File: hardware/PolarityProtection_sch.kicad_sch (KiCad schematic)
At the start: 14 parts, among them IC1 LM74502HDDFR, Q4 PSMN8R5-40MSDX

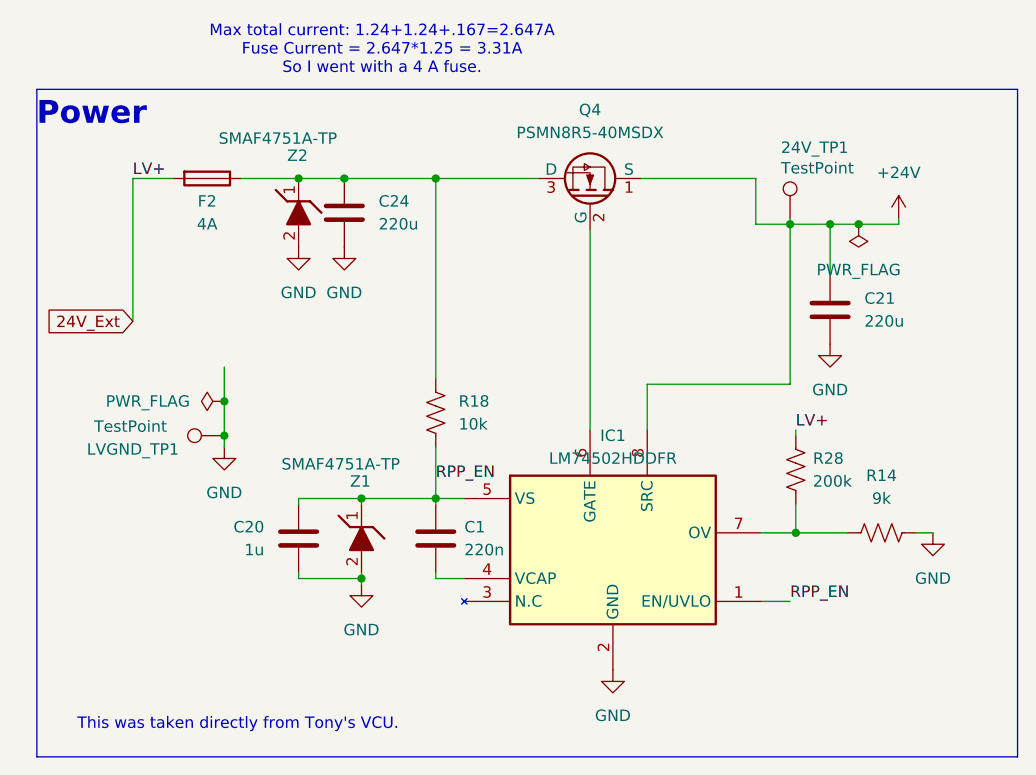
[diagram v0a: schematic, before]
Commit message: BOM
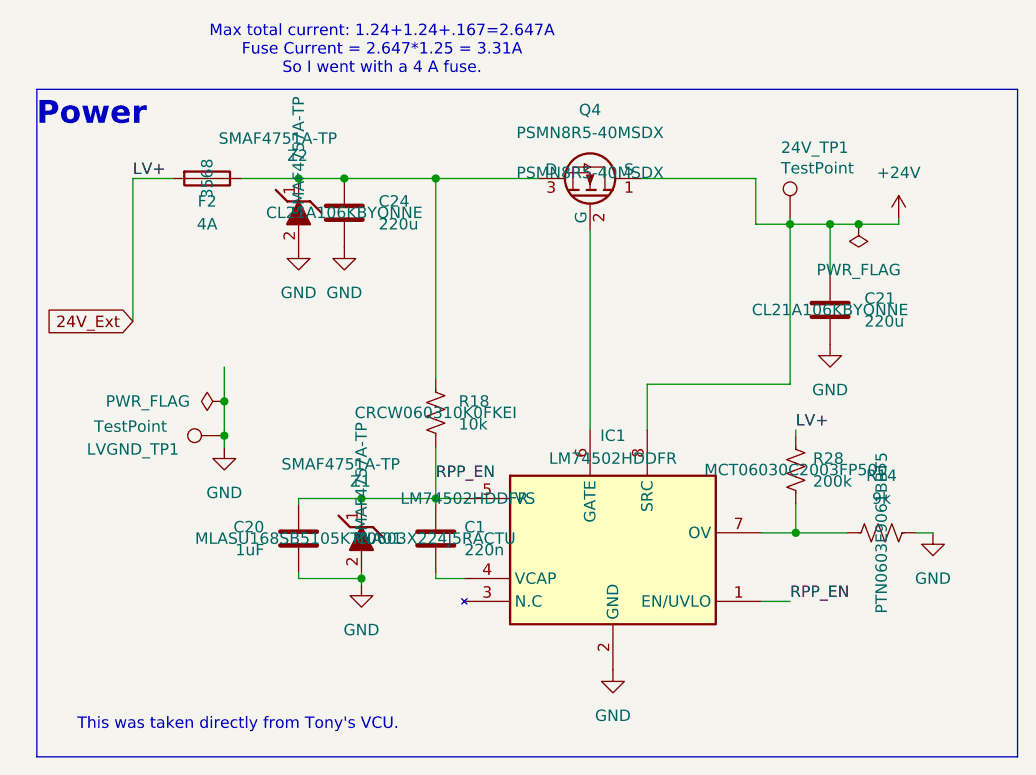
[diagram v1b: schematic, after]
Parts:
- C1: P/N (none) -> C0603X224J5RACTU
- C20: value 1u -> 1uF; P/N (none) -> MLASU168SB5105KTNA01
- C21, C24: P/N (none) -> CL21A106KBYQNNE
- F2: P/N (none) -> 3568
- IC1: P/N (none) -> LM74502HDDFR
- Q4: P/N (none) -> PSMN8R5-40MSDX
- R14: P/N (none) -> PTN0603E9061BBT5
- R18: P/N (none) -> CRCW060310K0FKEI
- R28: P/N (none) -> MCT06030C2003FP500
- Z1, Z2: P/N (none) -> SMAF4757A-TP
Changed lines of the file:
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@@
 			)
 		)
-		(property "Description" "Unpolarized capacitor"
+		(property "Description" "Multilayer Ceramic Capacitors MLCC - SMD/SMT 50V 0.22uF X7R 125C 0603"
 			(at 122.555 92.075 0)
 			(effects
@@
 				)
 				(hide yes)
+			)
+		)
+		(property "P/N" "C0603X224J5RACTU"
+			(at 122.555 92.075 0)
+			(effects
+				(font
+					(size 1.27 1.27)
+				)
 			)
 		)
@@
 			)
 		)
-		(property "Description" "Resistor, US symbol"
+		(property "Description" "Thick Film Resistors - SMD 10K OHM 1%"
 			(at 122.555 78.105 0)
 			(effects
@@
 				)
 				(hide yes)
+			)
+		)
+		(property "P/N" "CRCW060310K0FKEI "
+			(at 122.555 78.105 0)
+			(effects
+				(font
+					(size 1.27 1.27)
+				)
 			)
 		)
@@
 			)
 		)
-		(property "Description" "Unpolarized capacitor"
+		(property "Description" "Multilayer Ceramic Capacitors MLCC - SMD/SMT 10uF 50V X5R 2012 0805"
 			(at 112.395 55.88 0)
 			(effects
@@
 				)
 				(hide yes)
+			)
+		)
+		(property "P/N" "CL21A106KBYQNNE"
+			(at 112.395 55.88 0)
+			(effects
+				(font
+					(size 1.27 1.27)
+				)
 			)
 		)
@@
 			)
 		)
-		(property "Description" "Fuse"
+		(property "Description" "THT Blade fuse holder"
 			(at 97.155 52.07 0)
 			(effects
@@
 				)
 				(hide yes)
+			)
+		)
+		(property "P/N" "3568"
+			(at 97.155 52.07 0)
+			(effects
+				(font
+					(size 1.27 1.27)
+				)
 			)
 		)
@@
 			)
 		)
-		(property "Description" "Hot Swap Voltage Controllers 3.2-V to 65-V industrial RPP controller with load disconnect, OVP, and high gate drive"
+		(property "Description" "Hot Swap Voltage Controllers 3.2-V to 65-V indust rial RPP controller"
 			(at 125.73 87.63 0)
 			(effects
@@
 				(justify left top)
 				(hide yes)
+			)
+		)
+		(property "P/N" "LM74502HDDFR"
+			(at 125.73 87.63 0)
+			(effects
+				(font
+					(size 1.27 1.27)
+				)
 			)
 		)
@@
 			)
 		)
-		(property "Description" "1.0 Watt Zener Diodes 6.2V to 100V"
+		(property "Description" "Zener Diodes ZENER DIODES,1W 51V, DO-221AC"
 			(at 107.315 49.53 0)
 			(effects
@@
 			)
 		)
+		(property "P/N" "SMAF4757A-TP"
+			(at 107.315 49.53 0)
+			(effects
+				(font
+					(size 1.27 1.27)
+				)
+			)
+		)
 		(pin "1"
 		)
@@
 			)
 		)
-		(property "Description" "1.0 Watt Zener Diodes 6.2V to 100V"
+		(property "Description" "Zener Diodes ZENER DIODES,1W 51V, DO-221AC"
 			(at 114.3 85.725 0)
 			(effects
@@
 				(justify left top)
 				(hide yes)
+			)
+		)
+		(property "P/N" "SMAF4757A-TP"
+			(at 114.3 85.725 0)
+			(effects
+				(font
+					(size 1.27 1.27)
+				)
 			)
 		)
@@
 			)
 		)
-		(property "Description" "Resistor, US symbol"
+		(property "Description" "Thin Film Resistors - SMD 9.06K OHM .1% 25PPM 1/6W"
 			(at 172.085 91.44 0)
 			(effects
@@
 				)
 				(hide yes)
+			)
+		)
+		(property "P/N" "PTN0603E9061BBT5"
+			(at 172.085 91.44 0)
+			(effects
+				(font
+					(size 1.27 1.27)
+				)
 			)
 		)
@@
 			)
 		)
-		(property "Description" "Unpolarized capacitor"
+		(property "Description" "Multilayer Ceramic Capacitors MLCC - SMD/SMT 10uF 50V X5R 2012 0805"
 			(at 166.37 66.675 0)
 			(effects
@@
 				)
 				(hide yes)
+			)
+		)
+		(property "P/N" "CL21A106KBYQNNE"
+			(at 166.37 66.675 0)
+			(effects
+				(font
+					(size 1.27 1.27)
+				)
 			)
 		)
@@
 			)
 		)
-		(property "Description" "MOSFETs PSMN8R5-40MSD/SOT1210/mLFPAK"
+		(property "Description" "MOSFETs SOT1210 N-CH 40V 60A"
 			(at 138.684 40.005 0)
 			(effects
@@
 				(justify left top)
 				(hide yes)
+			)
+		)
+		(property "P/N" "PSMN8R5-40MSDX"
+			(at 139.7 51.435 0)
+			(effects
+				(font
+					(size 1.27 1.27)
+				)
 			)
 		)
@@
 			)
 		)
-		(property "Value" "1u"
+		(property "Value" "1uF"
 			(at 103.505 93.3449 0)
 			(effects
@@
 			)
 		)
-		(property "Description" "Unpolarized capacitor"
+		(property "Description" "Multilayer Ceramic Capacitors MLCC - SMD/SMT 50V 1uF X5R 0603 10%"
 			(at 107.315 92.075 0)
 			(effects
@@
 				)
 				(hide yes)
+			)
+		)
+		(property "P/N" "MLASU168SB5105KTNA01"
+			(at 107.315 92.075 0)
+			(effects
+				(font
+					(size 1.27 1.27)
+				)
 			)
 		)
@@
 			)
 		)
-		(property "Description" "Resistor, US symbol"
+		(property "Description" "Thin Film Resistors - SMD .1W 200Kohm 1% 0603 50ppm Auto"
 			(at 162.56 84.455 0)
 			(effects
@@
 			)
 		)
+		(property "P/N" "MCT06030C2003FP500 "
+			(at 162.56 84.455 0)
+			(effects
+				(font
+					(size 1.27 1.27)
+				)
+			)
+		)

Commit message: RevA
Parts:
- F2: footprint Fuse:3588 -> Fuse:Fuseholder_Blade_Mini_Keystone_3568
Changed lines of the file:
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@@
 			)
 		)
-		(property "Footprint" "Fuse:3588"
+		(property "Footprint" "Fuse:Fuseholder_Blade_Mini_Keystone_3568"
 			(at 97.155 50.292 90)
 			(effects
